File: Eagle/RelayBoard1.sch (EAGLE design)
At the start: 12 parts, among them IC1 ULN2003AN, K1 4052, K2 4052, K3 4051, X1 MKDSN1,5/6-5,08, X2 MKDSN1,5/6-5,08, X3 Con1, X4 MKDSN1,5/3-5,08, X7 Con2

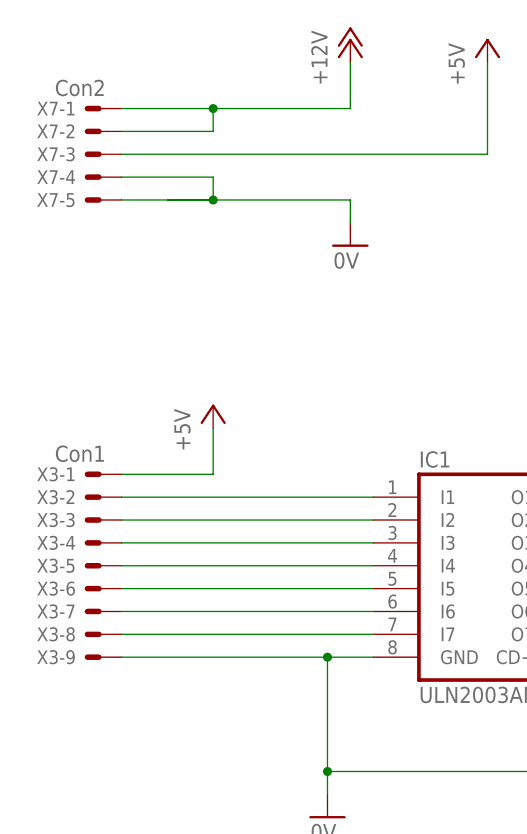
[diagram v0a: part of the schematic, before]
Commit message: - some modifications, corrections, ...
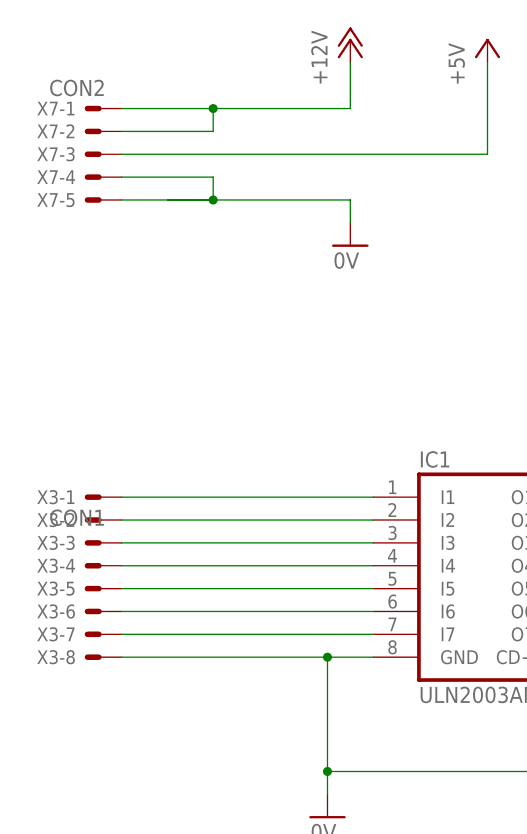
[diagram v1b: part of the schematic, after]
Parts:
- X3: value Con1 -> CON1; device con-molex:KK-156-9 -> con-molex:KK-156-8
- X7: value Con2 -> CON2
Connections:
- net +5V: no longer X3-1.S
- net 0V: now also X3-8.S; no longer X3-9.S
- net N$18: now also X3-1.S; no longer X3-2.S
- net N$19: now also X3-2.S; no longer X3-3.S
- net N$20: now also X3-3.S; no longer X3-4.S
- net N$21: now also X3-4.S; no longer X3-5.S
- net N$22: now also X3-5.S; no longer X3-6.S
- net N$23: now also X3-6.S; no longer X3-7.S
- net N$24: now also X3-7.S; no longer X3-8.S
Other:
- moved on the sheet: X3-1, X3-2, X3-3, X3-4, X3-5, X3-6, X3-7, X3-8
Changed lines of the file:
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@@
 </layers>
 <schematic xreflabel="%F%N/%S.%C%R" xrefpart="/%S.%C%R">
+<description>Main relay unit</description>
 <attributes>
 </attributes>
@@
 <part name="GND1" library="supply1" deviceset="0V" device=""/>
 <part name="GND2" library="supply1" deviceset="0V" device=""/>
-<part name="P+4" library="supply1" deviceset="+5V" device=""/>
 <part name="P+5" library="supply1" deviceset="+12V" device=""/>
 <part name="P+6" library="supply1" deviceset="+12V" device=""/>
 <part name="P+7" library="supply1" deviceset="+12V" device=""/>
 <part name="P+3" library="supply1" deviceset="+12V" device=""/>
-<part name="X3" library="con-molex" deviceset="KK-156-9" device="" value="Con1"/>
-<part name="X7" library="con-molex" deviceset="KK-156-5" device="" value="Con2"/>
+<part name="X7" library="con-molex" deviceset="KK-156-5" device="" value="CON2"/>
 <part name="X8" library="con-molex" deviceset="KK-156-3" device=""/>
 <part name="X9" library="con-molex" deviceset="KK-156-3" device=""/>
@@
 <attribute name="OC_NEWARK" value="70R0299"/>
 </part>
+<part name="X3" library="con-molex" deviceset="KK-156-8" device="" value="CON1"/>
 </parts>
 <sheets>
 <sheet>
-<description>RotorControl</description>
+<description>RotorControl - main relay board</description>
 <plain>
 </plain>
@@
 <instance part="GND1" gate="1" x="43.18" y="147.32"/>
 <instance part="GND2" gate="1" x="40.64" y="83.82"/>
-<instance part="P+4" gate="1" x="27.94" y="129.54"/>
 <instance part="P+5" gate="1" x="162.56" y="167.64"/>
 <instance part="P+6" gate="1" x="182.88" y="124.46"/>
 <instance part="P+7" gate="1" x="182.88" y="91.44"/>
 <instance part="P+3" gate="1" x="78.74" y="129.54"/>
-<instance part="X3" gate="-1" x="15.24" y="121.92" rot="MR0"/>
-<instance part="X3" gate="-2" x="15.24" y="119.38" rot="MR0"/>
-<instance part="X3" gate="-3" x="15.24" y="116.84" rot="MR0"/>
-<instance part="X3" gate="-4" x="15.24" y="114.3" rot="MR0"/>
-<instance part="X3" gate="-5" x="15.24" y="111.76" rot="MR0"/>
-<instance part="X3" gate="-6" x="15.24" y="109.22" rot="MR0"/>
-<instance part="X3" gate="-7" x="15.24" y="106.68" rot="MR0"/>
-<instance part="X3" gate="-8" x="15.24" y="104.14" rot="MR0"/>
-<instance part="X3" gate="-9" x="15.24" y="101.6" rot="MR0"/>
 <instance part="X7" gate="-1" x="15.24" y="162.56" rot="MR0"/>
 <instance part="X7" gate="-2" x="15.24" y="160.02" rot="MR0"/>
@@
 <instance part="X4" gate="-2" x="246.38" y="165.1"/>
 <instance part="X4" gate="-3" x="246.38" y="160.02"/>
+<instance part="X3" gate="-1" x="15.24" y="119.38" rot="R180"/>
+<instance part="X3" gate="-2" x="15.24" y="116.84" rot="R180"/>
+<instance part="X3" gate="-3" x="15.24" y="114.3" rot="R180"/>
+<instance part="X3" gate="-4" x="15.24" y="111.76" rot="R180"/>
+<instance part="X3" gate="-5" x="15.24" y="109.22" rot="R180"/>
+<instance part="X3" gate="-6" x="15.24" y="106.68" rot="R180"/>
+<instance part="X3" gate="-7" x="15.24" y="104.14" rot="R180"/>
+<instance part="X3" gate="-8" x="15.24" y="101.6" rot="R180"/>
 </instances>
 <busses>
@@
 </net>
 <net name="+5V" class="0">
-<segment>
-<pinref part="P+4" gate="1" pin="+5V"/>
-<wire x1="27.94" y1="121.92" x2="27.94" y2="127" width="0.1524" layer="91"/>
-<pinref part="X3" gate="-1" pin="S"/>
-<wire x1="17.78" y1="121.92" x2="27.94" y2="121.92" width="0.1524" layer="91"/>
-</segment>
 <segment>
 <wire x1="17.78" y1="157.48" x2="58.42" y2="157.48" width="0.1524" layer="91"/>
@@
 <wire x1="40.64" y1="101.6" x2="17.78" y2="101.6" width="0.1524" layer="91"/>
 <junction x="40.64" y="101.6"/>
-<pinref part="X3" gate="-9" pin="S"/>
 <pinref part="GND2" gate="1" pin="0V"/>
 <wire x1="40.64" y1="86.36" x2="40.64" y2="88.9" width="0.1524" layer="91"/>
 <junction x="40.64" y="88.9"/>
+<pinref part="X3" gate="-8" pin="S"/>
 </segment>
 </net>
@@
 <pinref part="IC1" gate="A" pin="I1"/>
 <wire x1="45.72" y1="119.38" x2="17.78" y2="119.38" width="0.1524" layer="91"/>
-<pinref part="X3" gate="-2" pin="S"/>
+<pinref part="X3" gate="-1" pin="S"/>
 </segment>
 </net>
@@
 <pinref part="IC1" gate="A" pin="I2"/>
 <wire x1="45.72" y1="116.84" x2="17.78" y2="116.84" width="0.1524" layer="91"/>
-<pinref part="X3" gate="-3" pin="S"/>
+<pinref part="X3" gate="-2" pin="S"/>
 </segment>
 </net>
@@
 <pinref part="IC1" gate="A" pin="I3"/>
 <wire x1="45.72" y1="114.3" x2="17.78" y2="114.3" width="0.1524" layer="91"/>
-<pinref part="X3" gate="-4" pin="S"/>
+<pinref part="X3" gate="-3" pin="S"/>
 </segment>
 </net>
@@
 <pinref part="IC1" gate="A" pin="I4"/>
 <wire x1="45.72" y1="111.76" x2="17.78" y2="111.76" width="0.1524" layer="91"/>
-<pinref part="X3" gate="-5" pin="S"/>
+<pinref part="X3" gate="-4" pin="S"/>
 </segment>
 </net>
@@
 <pinref part="IC1" gate="A" pin="I5"/>
 <wire x1="45.72" y1="109.22" x2="17.78" y2="109.22" width="0.1524" layer="91"/>
-<pinref part="X3" gate="-6" pin="S"/>
+<pinref part="X3" gate="-5" pin="S"/>
 </segment>
 </net>
@@
 <pinref part="IC1" gate="A" pin="I6"/>
 <wire x1="45.72" y1="106.68" x2="17.78" y2="106.68" width="0.1524" layer="91"/>
-<pinref part="X3" gate="-7" pin="S"/>
+<pinref part="X3" gate="-6" pin="S"/>
 </segment>
 </net>
@@
 <pinref part="IC1" gate="A" pin="I7"/>
 <wire x1="45.72" y1="104.14" x2="17.78" y2="104.14" width="0.1524" layer="91"/>
-<pinref part="X3" gate="-8" pin="S"/>
-</segment>
-</net>
+<pinref part="X3" gate="-7" pin="S"/>
+</segment>
+</net>
